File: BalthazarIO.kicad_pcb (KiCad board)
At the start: 2 copper layers, 112 x 30.2 mm, 70 parts, among them J1 USB_B_Micro, J10 USB_01x04, J11 USB_01x04, J2 Conn_01x04_Female, J3 USB_A, J4 USB_A, J5 USB_A, J6 USB_A, J7 Conn_01x04_Male, J8 USB_01x04, J9 USB_01x04, SW1 SW_DIP_x01, SW2 SW_DIP_x01, SW3 SW_DIP_x01, SW4 SW_DIP_x01, U1 GL850G-28pin, U2 AT24CS02-XHM, U3 AIC1526-0, U4 AIC1526-0, Y1 Crystal 12MHz

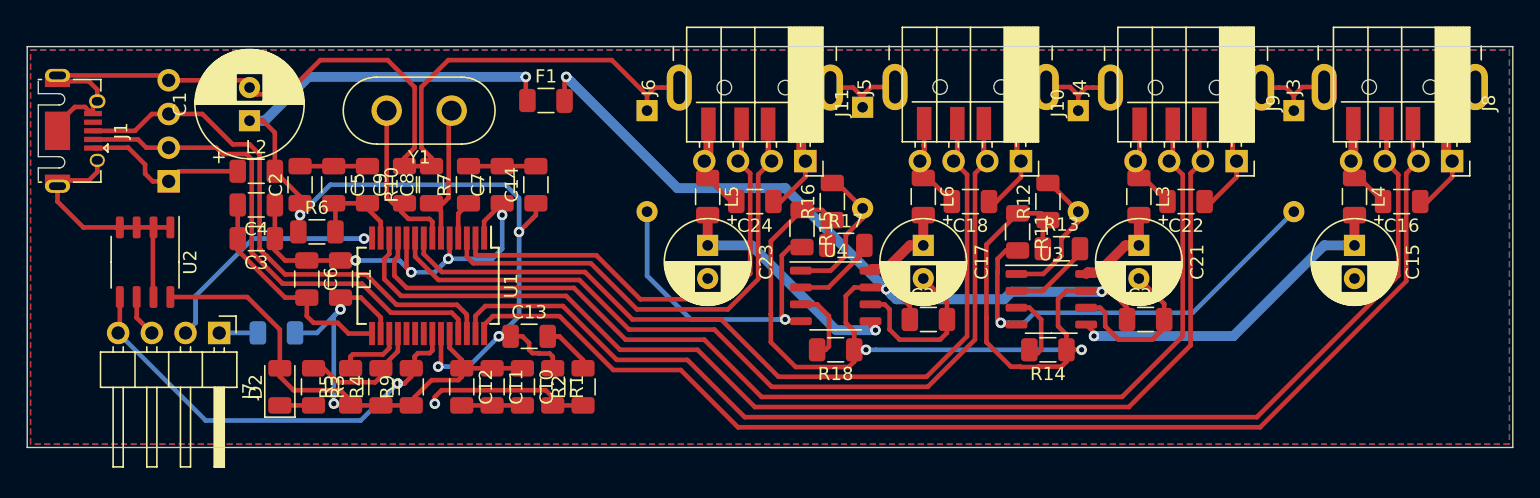
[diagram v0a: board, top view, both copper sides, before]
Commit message: Add files via upload
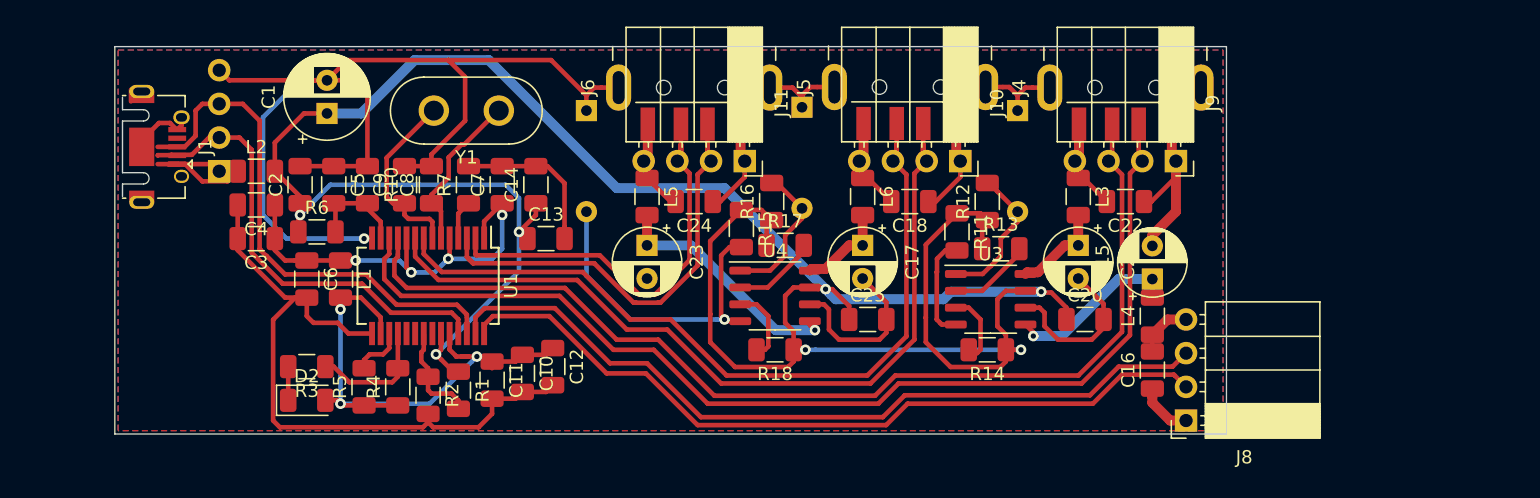
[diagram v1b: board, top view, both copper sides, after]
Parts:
- removed C19: 100n, Capacitor_SMD:C_1206_3216Metric
- removed F1: 500mA, Fuse:Fuse_1206_3216Metric
- removed J3: USB_A, Connector_USB:USB_A_CNCTech_1001-011-01101_Horizontal
- removed J7: Conn_01x04_Male, Connector_PinHeader_2.54mm:PinHeader_1x04_P2.54mm_Horizontal
- removed R9: 10K, Resistor_SMD:R_1206_3216Metric
- removed SW1: SW_DIP_x01, Button_Switch_THT:SW_DIP_SPSTx01_Slide_9.78x4.72mm_W7.62mm_P2.54mm
- removed U2: AT24CS02-XHM, Package_SO:SOP-8_3.9x4.9mm_P1.27mm
- C1: footprint Capacitor_THT:CP_Radial_D8.0mm_P2.50mm -> Capacitor_THT:CP_Radial_D6.3mm_P2.50mm
- C15: value 100uF -> 47uF; footprint Capacitor_THT:CP_Radial_D6.3mm_P2.50mm -> Capacitor_THT:CP_Radial_D5.0mm_P2.50mm
- C17, C21, C23: footprint Capacitor_THT:CP_Radial_D6.3mm_P2.50mm -> Capacitor_THT:CP_Radial_D5.0mm_P2.50mm
- J8: value USB_01x04 -> USB1.1 keyboard+touchpad
- moved J8 28.0 mm to (113.3, 99.1), turned to 180 degrees
- moved C16 22.7 mm to (110.7, 95.2), turned to 90 degrees
- moved L4 17.7 mm to (110.7, 91.2), turned to 90 degrees
- moved C15 15.5 mm to (110.7, 88.4), turned to 90 degrees
- moved R2 11.7 mm to (56.1, 97.2), turned to 270 degrees
- moved C13 7.47 mm to (65.0, 85.3)
- moved R1 7.12 mm to (58.4, 96.8)
- moved C12 7.03 mm to (65.5, 95.0)
- moved J1 6.46 mm to (34.5, 78.4)
- moved C1 5.87 mm to (48.5, 75.9)
- moved C18 4.57 mm to (92.5, 82.5)
- moved C20 4.57 mm to (105.7, 91.4)
- moved C22 4.57 mm to (108.7, 82.5)
- moved C24 4.57 mm to (76.2, 82.5)
- moved J4 4.57 mm to (108.7, 67.1)
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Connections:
- C20 pad 1: Net-(C20-Pad1) -> 5V
- C25 pad 1: Net-(C20-Pad1) -> 5V
- R11 pad 1: Net-(C20-Pad1) -> 5V
- R12 pad 1: Net-(C20-Pad1) -> 5V
- R13 pad 1: Net-(C20-Pad1) -> 5V
- R14 pad 1: Net-(C20-Pad1) -> 5V
- R15 pad 1: Net-(C20-Pad1) -> 5V
- R16 pad 1: Net-(C20-Pad1) -> 5V
- R17 pad 1: Net-(C20-Pad1) -> 5V
- R18 pad 1: Net-(C20-Pad1) -> 5V
- U1 pad 14: Net-(J7-Pad2) -> GND
- U1 pad 22: Net-(J7-Pad4) -> (no net)
- U3 pad 7: Net-(C20-Pad1) -> 5V
- U4 pad 7: Net-(C20-Pad1) -> 5V
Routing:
- net Net-(C20-Pad1): track 138.7 -> 0.00 mm, vias 5 -> 0
- net 5V: track 80.2 -> 203.6 mm, vias 5 -> 7
- net Net-(J7-Pad4): track 33.3 -> 0.00 mm, vias 1 -> 0
- net Net-(J8-Pad2): track 91.3 -> 59.2 mm
- net Net-(J8-Pad3): track 91.4 -> 60.5 mm
- net Net-(R11-Pad2): track 33.5 -> 7.94 mm, vias 1 -> 0
- net Net-(J7-Pad2): track 18.2 -> 0.00 mm, vias 1 -> 0
- net +3V3: track 56.0 -> 41.2 mm, vias 2 -> 3
- net Net-(C15-Pad1): track 25.9 -> 13.3 mm
- net GND: track 235.2 -> 241.5 mm, vias 0 -> 1
- net Net-(J11-Pad3): track 38.5 -> 33.1 mm
- net Net-(J4-Pad3): track 87.1 -> 81.9 mm
- net Net-(J11-Pad2): track 41.0 -> 35.9 mm
- net Net-(R1-Pad2): track 12.7 -> 7.79 mm, vias 1 -> 0
- net Net-(J4-Pad2): track 84.6 -> 79.8 mm
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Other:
- board size 112 x 30.2 mm -> 83.8 x 29.2 mm
